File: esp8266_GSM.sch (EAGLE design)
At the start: 15 parts, among them IC1 REG1117, Q2 220mA/50V/3.5Ω, Q4 220mA/50V/3.5Ω, Q5 220mA/50V/3.5Ω, U1 ESP8266-12E/ESP-12E

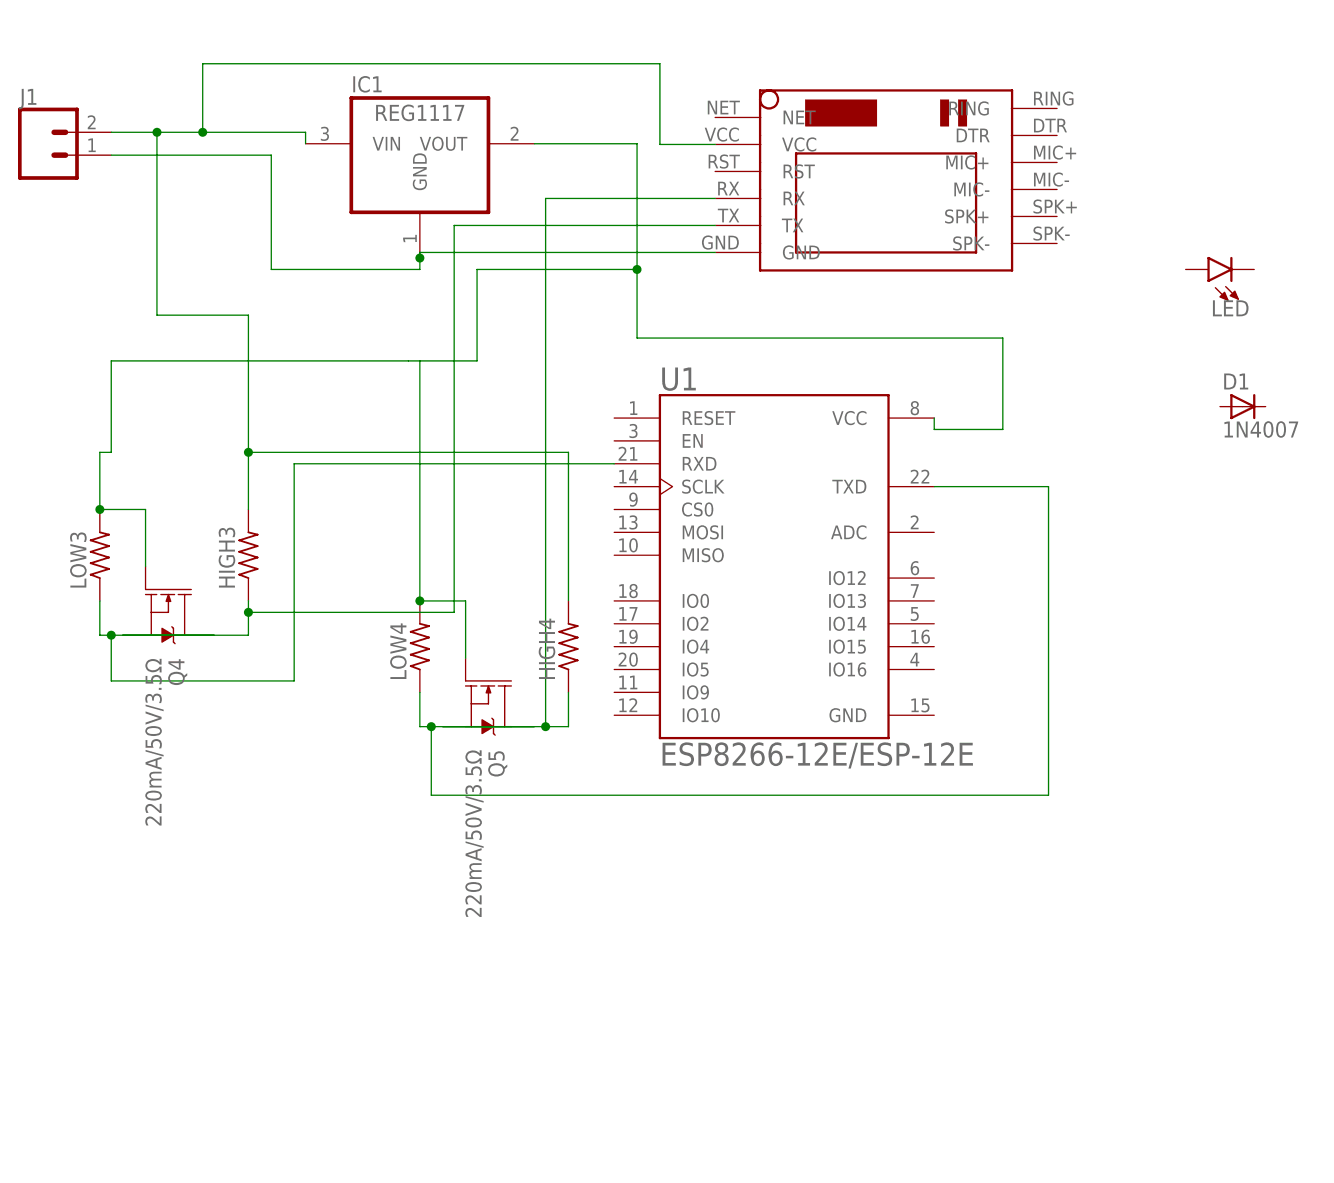
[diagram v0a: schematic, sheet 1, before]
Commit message: components added
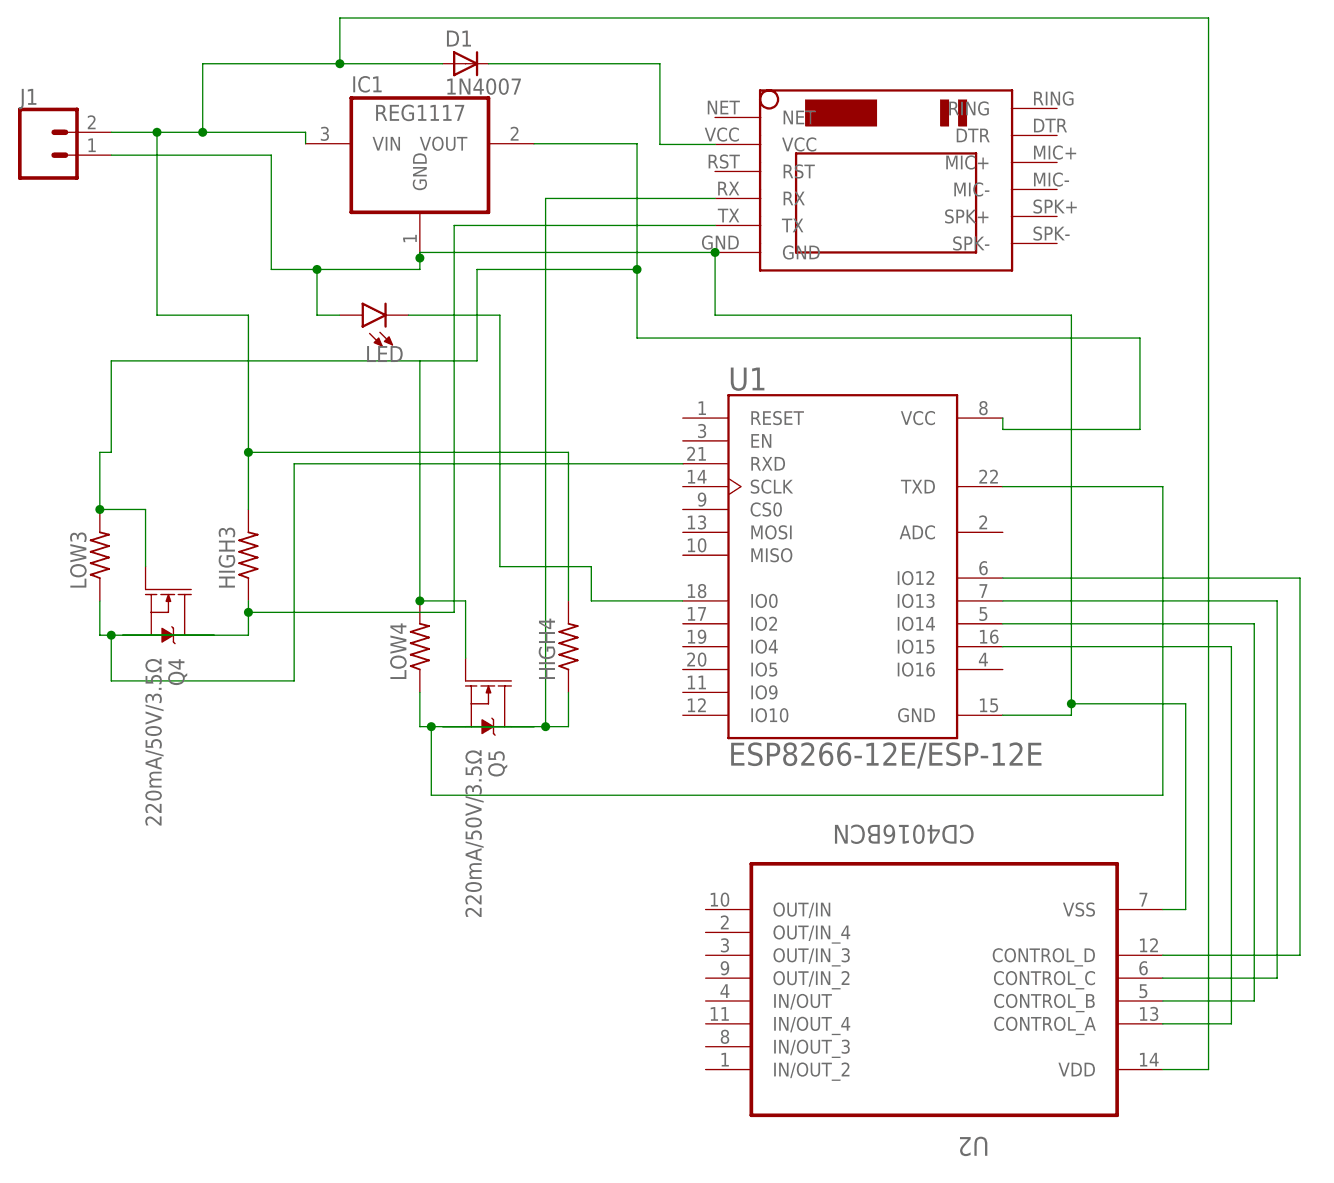
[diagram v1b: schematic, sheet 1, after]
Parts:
- added U2: CD4016BCN, CD4016BCN:CD4016BCN
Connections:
- removed net N$4: IC1.GND, J1.1, U$1.GND
- new net N$12: U1.IO14, U2.CONTROL_B
- new net N$16: U1.IO15, U2.CONTROL_A
- new net N$17: D1.A, HIGH3.2, HIGH4.2, IC1.VIN, J1.2, U2.VDD
- new net N$3: LED.C, U1.IO0
- new net N$5: D1.C, U$1.VCC
- new net N$7: U1.IO12, U2.CONTROL_D
- new net N$8: U1.IO13, U2.CONTROL_C
- net N$6: now also IC1.GND, J1.1, LED.A, U$1.GND, U1.GND, U2.VSS; no longer HIGH3.2, HIGH4.2, IC1.VIN, J1.2, U$1.VCC
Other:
- moved on the sheet: D1, LED, U1
